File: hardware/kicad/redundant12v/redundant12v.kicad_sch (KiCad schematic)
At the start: 23 parts, among them J1 Conn_01x06, J2 IDC 2x5 Male, Q1 2N3904, Q2 2N3904, U1 ATtiny212-SS, U2 MAX232CPE, U3 LD1117S50TR_SOT223, X1 ASCO

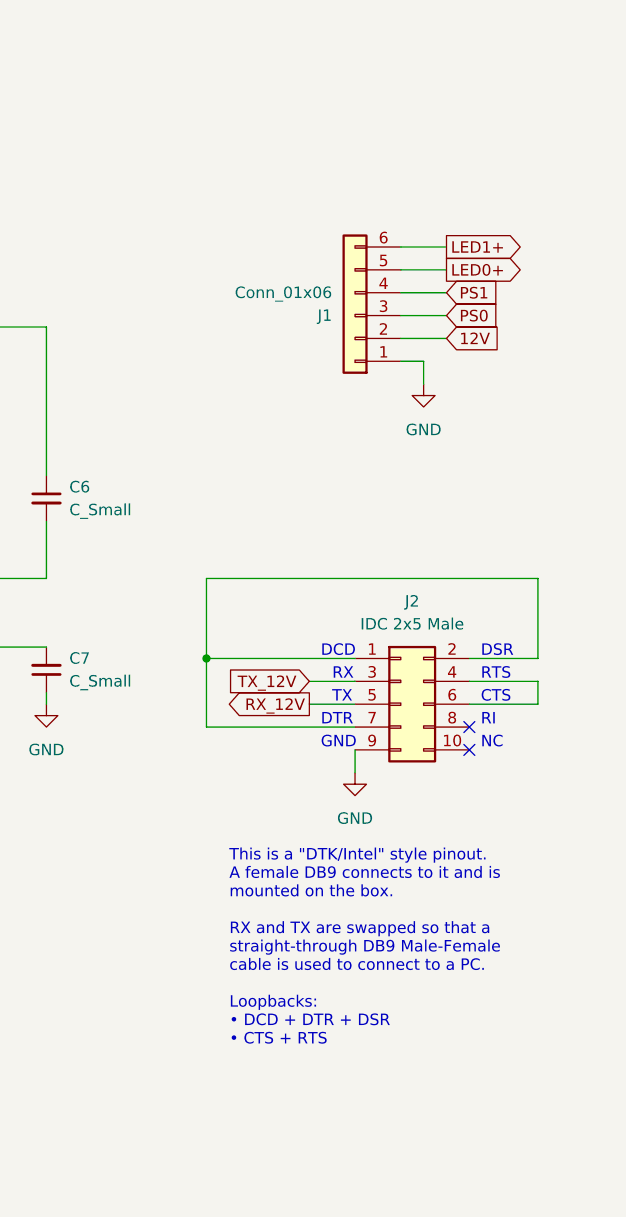
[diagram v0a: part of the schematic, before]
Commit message: PCB rev 1 finished
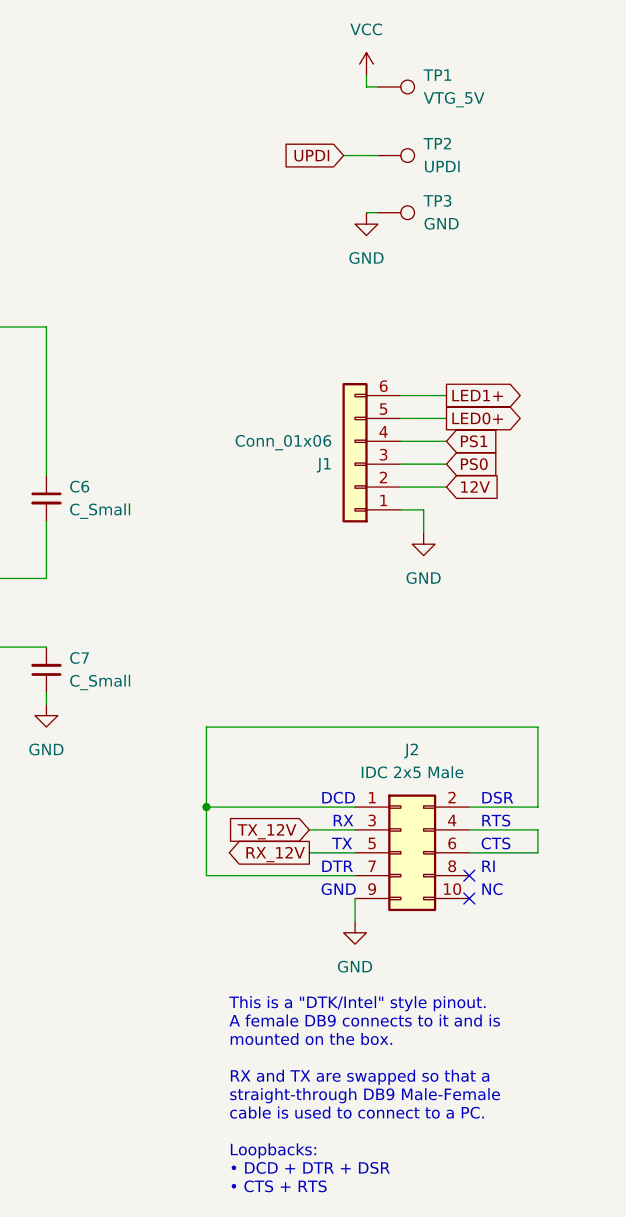
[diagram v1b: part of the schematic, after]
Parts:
- added TP1: VTG_5V, TestPoint:TestPoint_Pad_D2.5mm, symbol Connector:TestPoint
- added TP2: UPDI, TestPoint:TestPoint_Pad_D2.5mm, symbol Connector:TestPoint
- added TP3: GND, TestPoint:TestPoint_Pad_D2.5mm, symbol Connector:TestPoint
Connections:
- net GND: now also TP3.1
- net UPDI: now also TP2.1
- net VCC: now also TP1.1
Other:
- moved on the sheet: J1, J2
